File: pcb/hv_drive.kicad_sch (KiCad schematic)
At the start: 0 parts

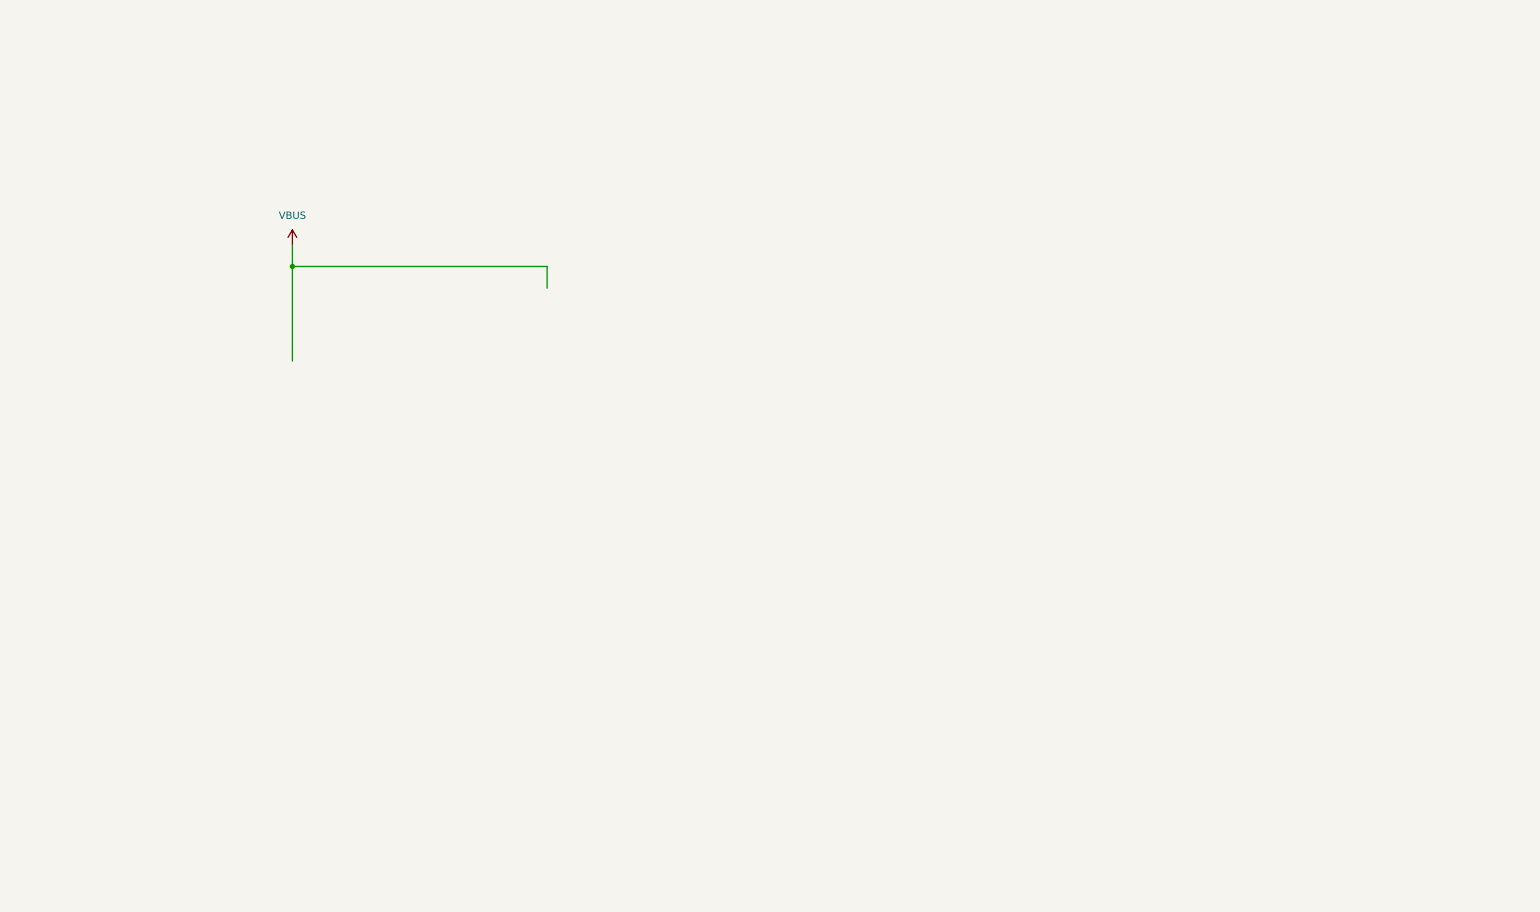
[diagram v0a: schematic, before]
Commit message: w
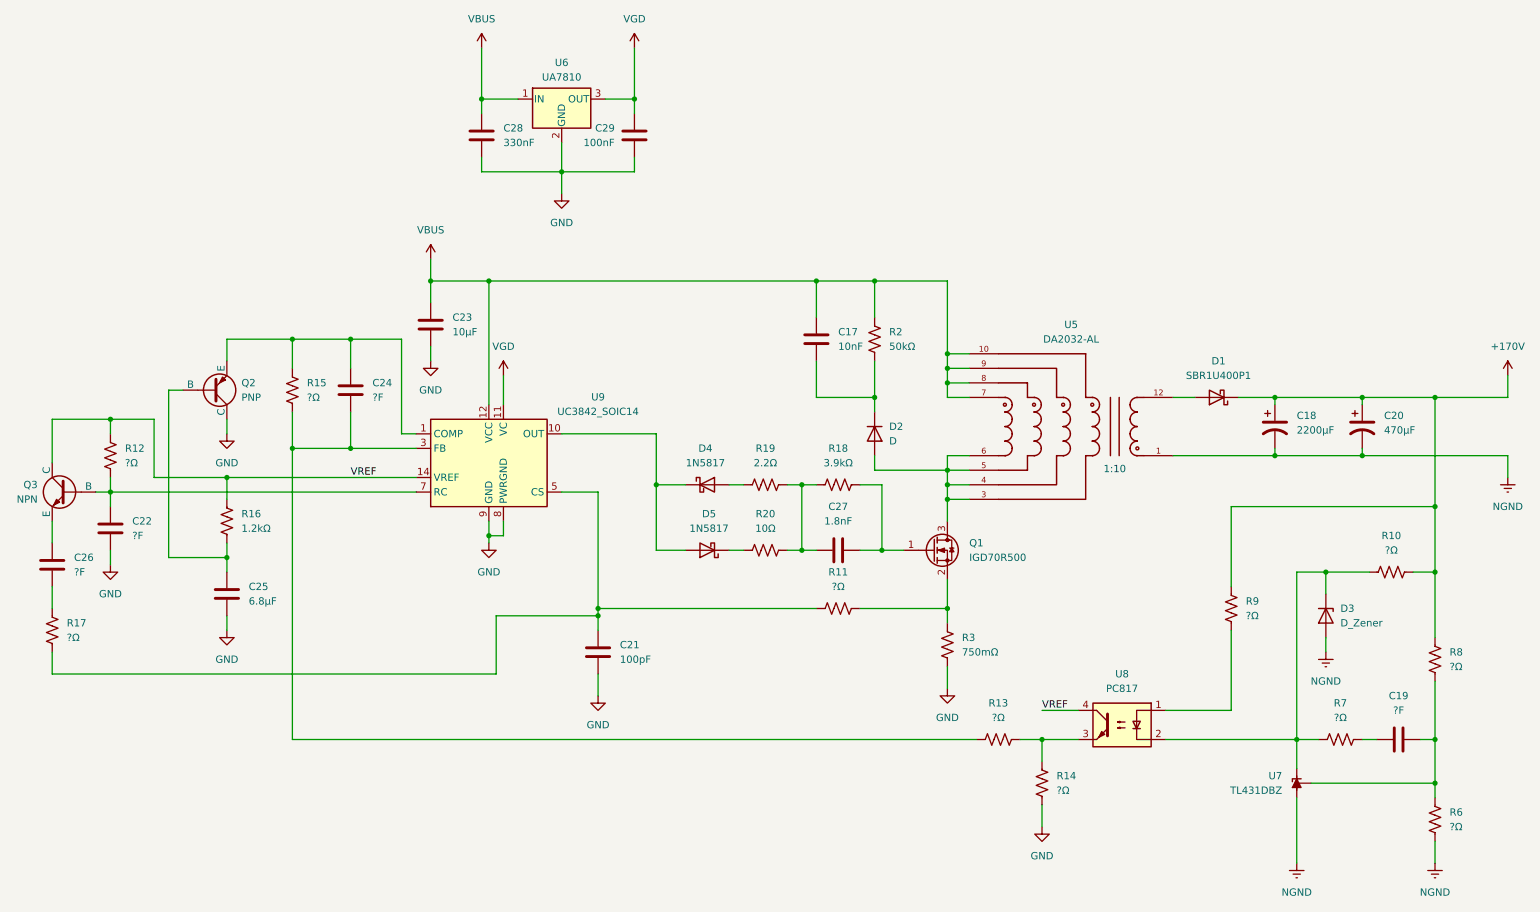
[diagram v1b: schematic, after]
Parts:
- added C17: 10nF, Capacitor_SMD:C_1206_3216Metric_Pad1.33x1.80mm_HandSolder, symbol Device:C
- added C18: 2200μF, Capacitor_SMD:C_1206_3216Metric_Pad1.33x1.80mm_HandSolder, symbol Device:C_Polarized_US
- added C19, C22, C24, C26: ?F, Capacitor_SMD:C_1206_3216Metric_Pad1.33x1.80mm_HandSolder, symbol Device:C
- added C20: 470μF, Capacitor_SMD:C_1206_3216Metric_Pad1.33x1.80mm_HandSolder, symbol Device:C_Polarized_US
- added C21: 100pF, Capacitor_SMD:C_1206_3216Metric_Pad1.33x1.80mm_HandSolder, symbol Device:C
- added C23: 10μF, Capacitor_SMD:C_1206_3216Metric_Pad1.33x1.80mm_HandSolder, symbol Device:C
- added C25: 6.8μF, Capacitor_SMD:C_1206_3216Metric_Pad1.33x1.80mm_HandSolder, symbol Device:C
- added C27: 1.8nF, Capacitor_SMD:C_1206_3216Metric_Pad1.33x1.80mm_HandSolder, symbol Device:C
- added C28: 330nF, Capacitor_SMD:C_1206_3216Metric_Pad1.33x1.80mm_HandSolder, symbol Device:C
- added C29: 100nF, Capacitor_SMD:C_1206_3216Metric_Pad1.33x1.80mm_HandSolder, symbol Device:C
- added D1: SBR1U400P1, symbol Device:D_Schottky
- added D2: D, symbol Device:D
- added D3: D_Zener, symbol Device:D_Zener
- added D4, D5: 1N5817, Diode_THT:D_DO-41_SOD81_P10.16mm_Horizontal, symbol Diode:1N5817
- added Q1: IGD70R500, Package_TO_SOT_SMD:TO-252-2, symbol Transistor_FET:Q_NMOS_GSD
- added Q2: PNP, symbol Simulation_SPICE:PNP
- added Q3: NPN, symbol Simulation_SPICE:NPN
- added R10, R11, R12, R13, R14, R15, R17, R6, R7, R8, R9: ?Ω, Resistor_SMD:R_1206_3216Metric_Pad1.30x1.75mm_HandSolder, symbol Device:R_US
- added R16: 1.2kΩ, Resistor_SMD:R_1206_3216Metric_Pad1.30x1.75mm_HandSolder, symbol Device:R_US
- added R18: 3.9kΩ, Resistor_SMD:R_1206_3216Metric_Pad1.30x1.75mm_HandSolder, symbol Device:R_US
- added R19: 2.2Ω, Resistor_SMD:R_1206_3216Metric_Pad1.30x1.75mm_HandSolder, symbol Device:R_US
- added R2: 50kΩ, Resistor_SMD:R_1206_3216Metric_Pad1.30x1.75mm_HandSolder, symbol Device:R_US
- added R20: 10Ω, Resistor_SMD:R_1206_3216Metric_Pad1.30x1.75mm_HandSolder, symbol Device:R_US
- added R3: 750mΩ, Resistor_SMD:R_1206_3216Metric_Pad1.30x1.75mm_HandSolder, symbol Device:R_US
- added U5: DA2032-AL, Footprints:DA2032-AL, symbol DA2032-AL:DA2032-AL
- added U6: UA7810, Package_TO_SOT_THT:TO-220-3_Vertical, symbol Regulator_Linear:uA7810
- added U7: TL431DBZ, Package_TO_SOT_SMD:SOT-23, symbol Reference_Voltage:TL431DBZ
- added U8: PC817, Package_DIP:DIP-4_W7.62mm, symbol Isolator:PC817
- added U9: UC3842_SOIC14, Package_SO:SOIC-14_3.9x8.7mm_P1.27mm, symbol Regulator_Controller:UC3842_SOIC14
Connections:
- net VBUS: now also C17.1, C23.1, C28.1, R2.1, U5.10, U5.7, U5.8, U5.9, U6.1 (IN), U9.12 (VCC)
- new net: C24.1, R13.1, R15.1, U9.3 (FB)
- new net: C24.2, Q2.3 (E), R15.2, U9.1 (COMP)
- new net: D1.2 (A), U5.12
- new net: D2.2 (A), Q1.3 (D), U5.3, U5.4, U5.5, U5.6
- new net: C17.2, D2.1 (K), R2.2
- new net: D3.1 (K), R10.1, R7.1, U7.1 (K), U8.2
- new net: C19.2, R6.1, R8.2, U7.2 (REF)
- new net: C25.2, Q2.2 (B), R16.1
- new net: D5.1 (K), R20.1
- new net: C27.1, R18.1, R19.2, R20.2
- new net: D4.2 (A), R19.1
- new net: C26.1, R17.2
- new net: C26.2, Q3.3 (E)
- new net: D4.1 (K), D5.2 (A), U9.10 (OUT)
- new net: C22.2, Q3.2 (B), R12.1, U9.7 (RC)
- new net: Q1.2 (S), R11.2, R3.1
- new net: C21.1, R11.1, R17.1, U9.5 (CS)
- new net: C27.2, Q1.1 (G), R18.2
- new net: C19.1, R7.2
- new net: R13.2, R14.2, U8.3
- new net: R9.2, U8.1
- new net +170V: C18.1, C20.1, D1.1 (K), R10.2, R8.1, R9.1
- new net GND: C21.2, C22.1, C23.2, C25.1, C28.2, C29.2, Q2.1 (C), R14.1, R3.2, U6.2 (GND), U9.8 (PWRGND), U9.9 (GND)
- new net NGND: C18.2, C20.2, D3.2 (A), R6.2, U5.1, U7.3 (A)
- new net VGD: C29.1, U6.3 (OUT), U9.11 (VC)
- new net VREF: Q3.1 (C), R12.2, R16.2, U8.4, U9.14 (VREF)
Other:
- note added: "1:10"
